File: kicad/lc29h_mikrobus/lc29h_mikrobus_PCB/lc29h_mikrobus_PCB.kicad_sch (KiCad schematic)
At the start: 6 parts, among them IC1 MIKROE-924, IC2 TXS0108EPWR, IC3 DS28E36BQ+U, IC4 74LVC1G3157GV,125

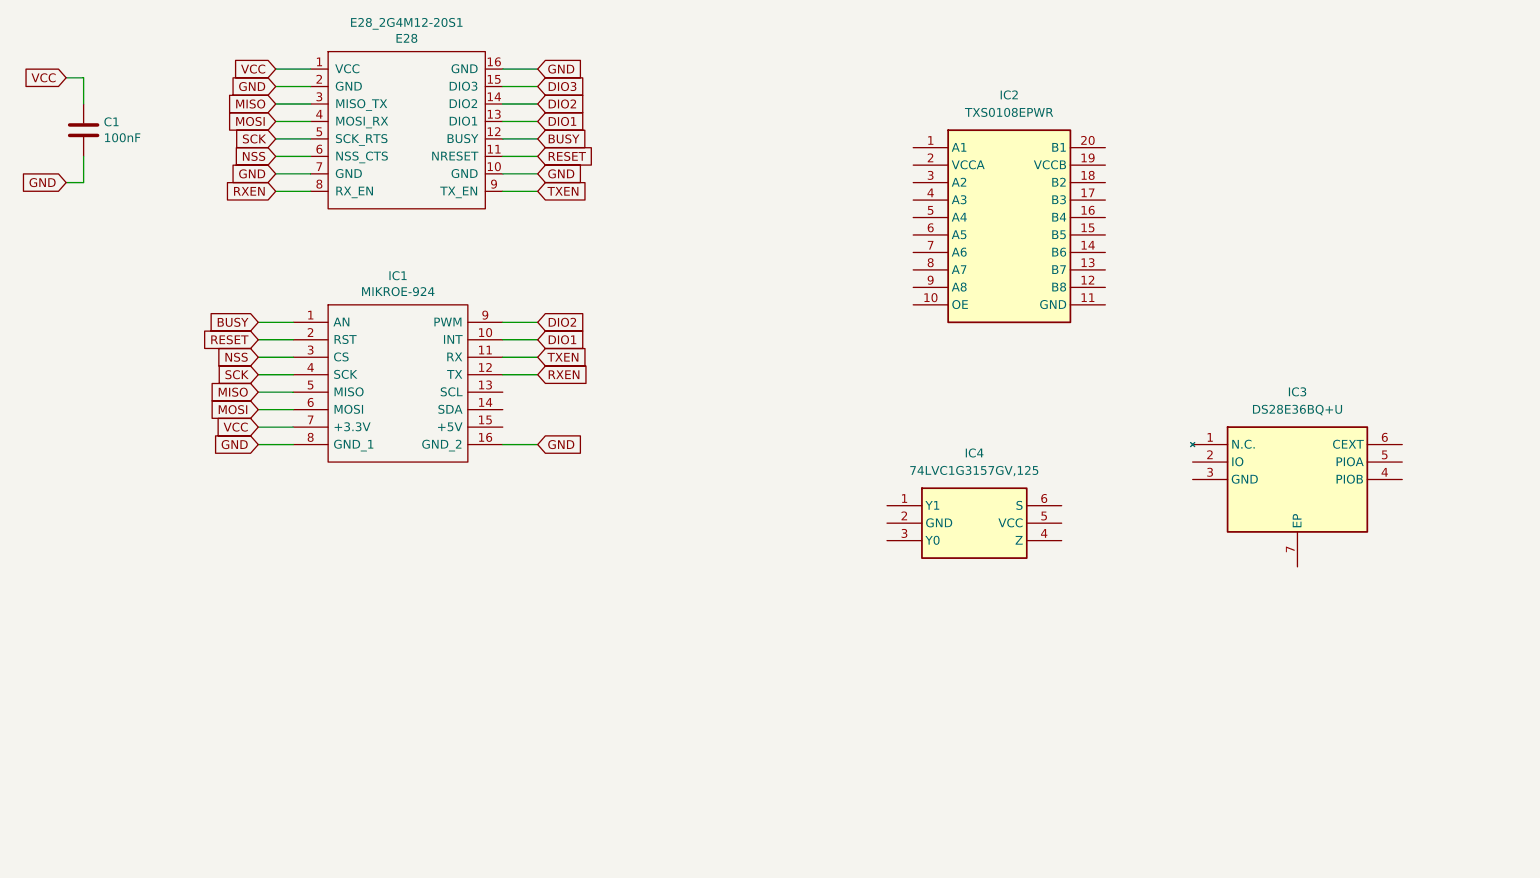
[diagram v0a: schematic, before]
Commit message: Début circuit
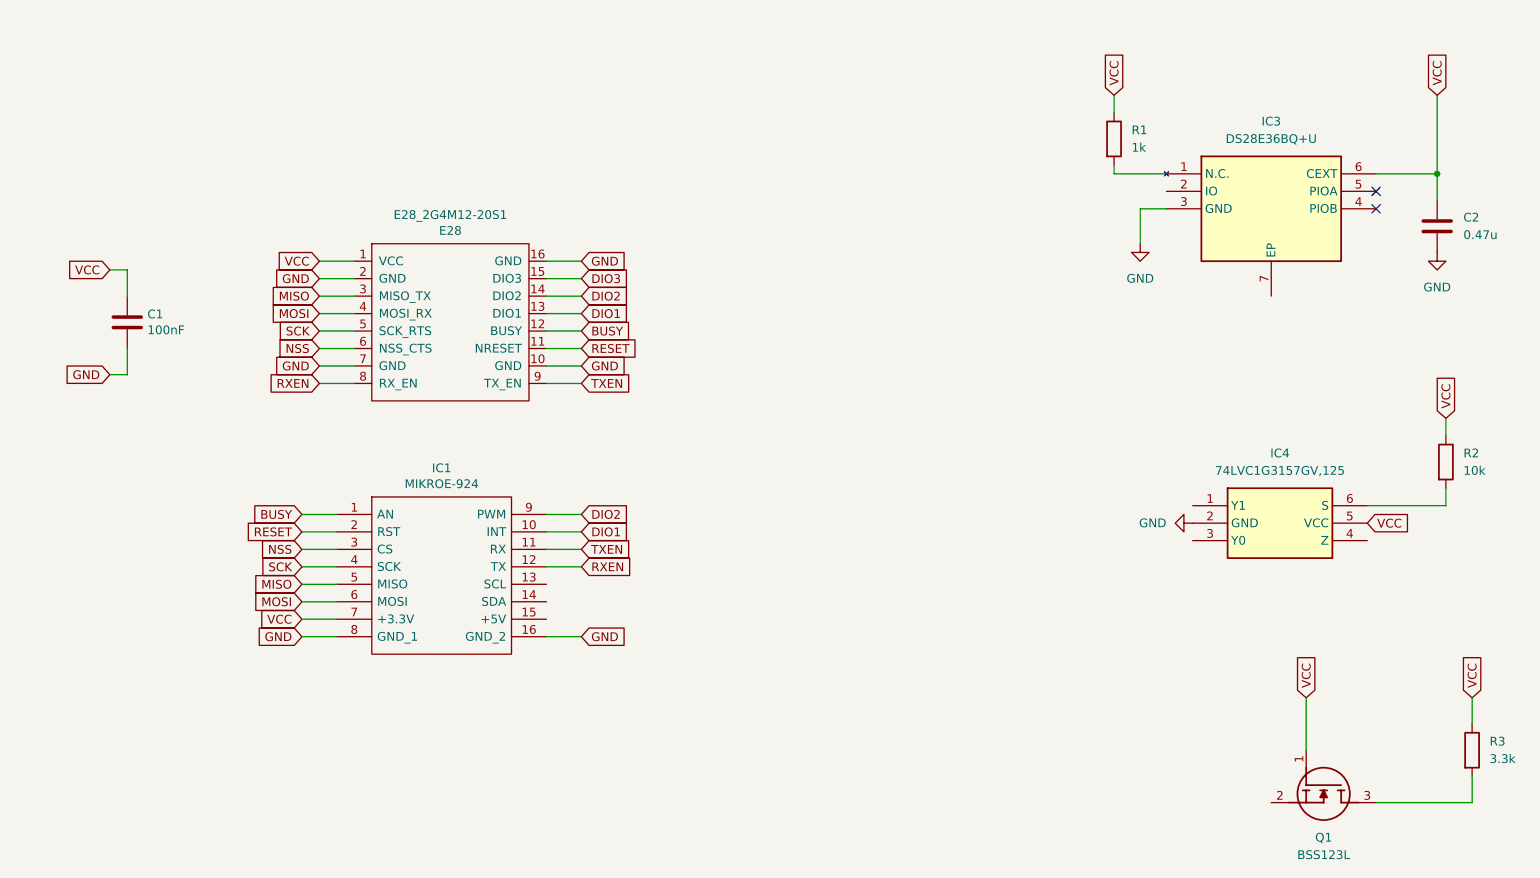
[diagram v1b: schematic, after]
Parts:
- removed IC2: TXS0108EPWR, SOP65P640X120-20N, symbol TXS0108EPWR:TXS0108EPWR
- added C2: 0.47u, symbol Device:C
- added Q1: BSS123L, SOT96P237X111-3N, symbol BSS123L:BSS123L
- added R1: 1k, symbol Device:R
- added R2: 10k, symbol Device:R
- added R3: 3.3k, symbol Device:R
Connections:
- net GND: now also IC3.3 (GND), IC4.2 (GND), C2.2
- net VCC: now also IC3.6 (CEXT), IC4.5 (VCC), C2.1, Q1.1 (G), R1.1, R2.1, R3.1
- net at IC4.6 (S): now also R2.2
- net at IC3.1 (N.C.): now also R1.2
- new net: Q1.3 (D), R3.2
- no-connect marks 0 -> 2
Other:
- moved on the sheet: C1, E28_2G4M12-20S1, IC1, IC3, IC4
